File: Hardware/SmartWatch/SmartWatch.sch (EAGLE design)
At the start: 1 part

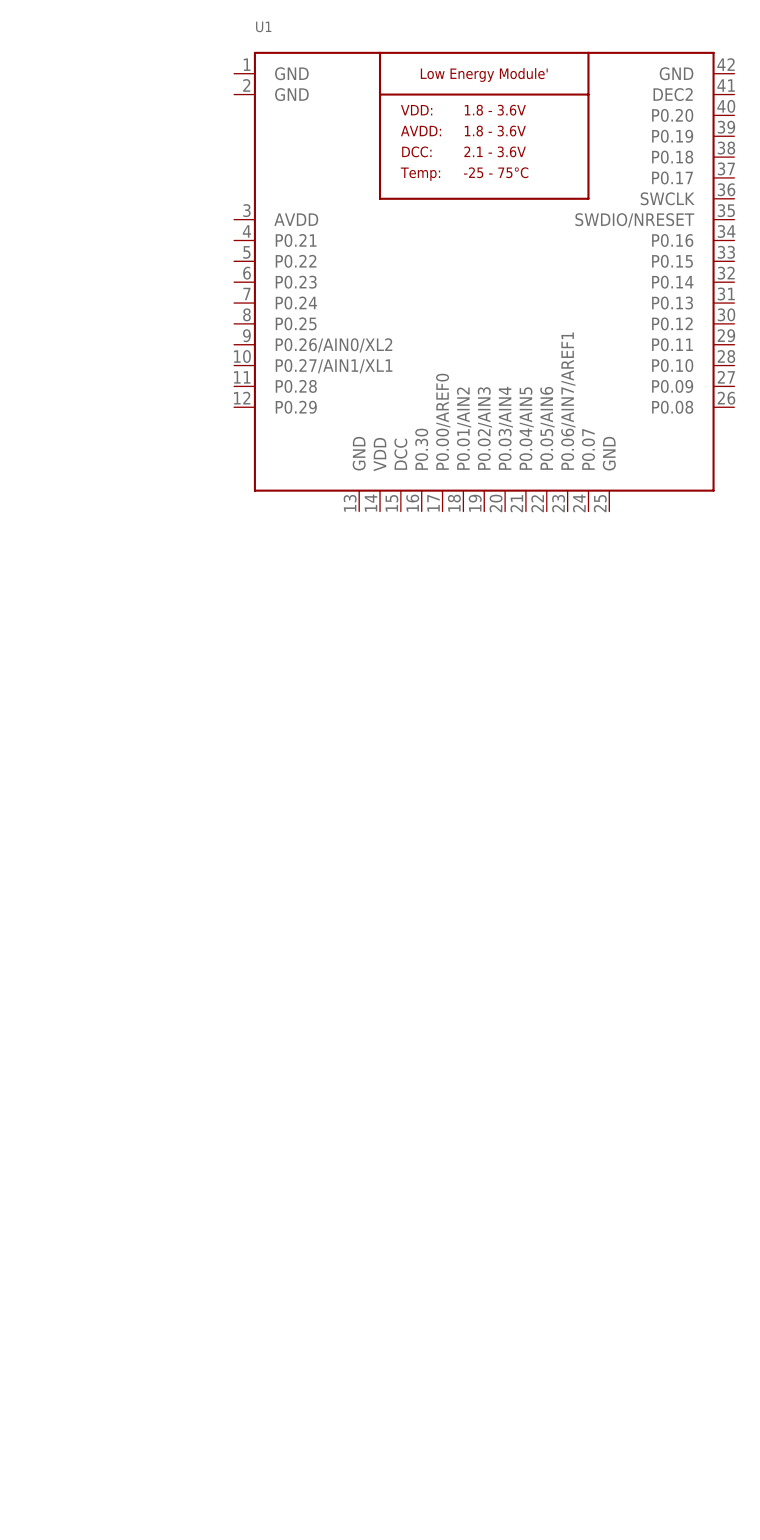
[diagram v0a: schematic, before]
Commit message: adding things to library
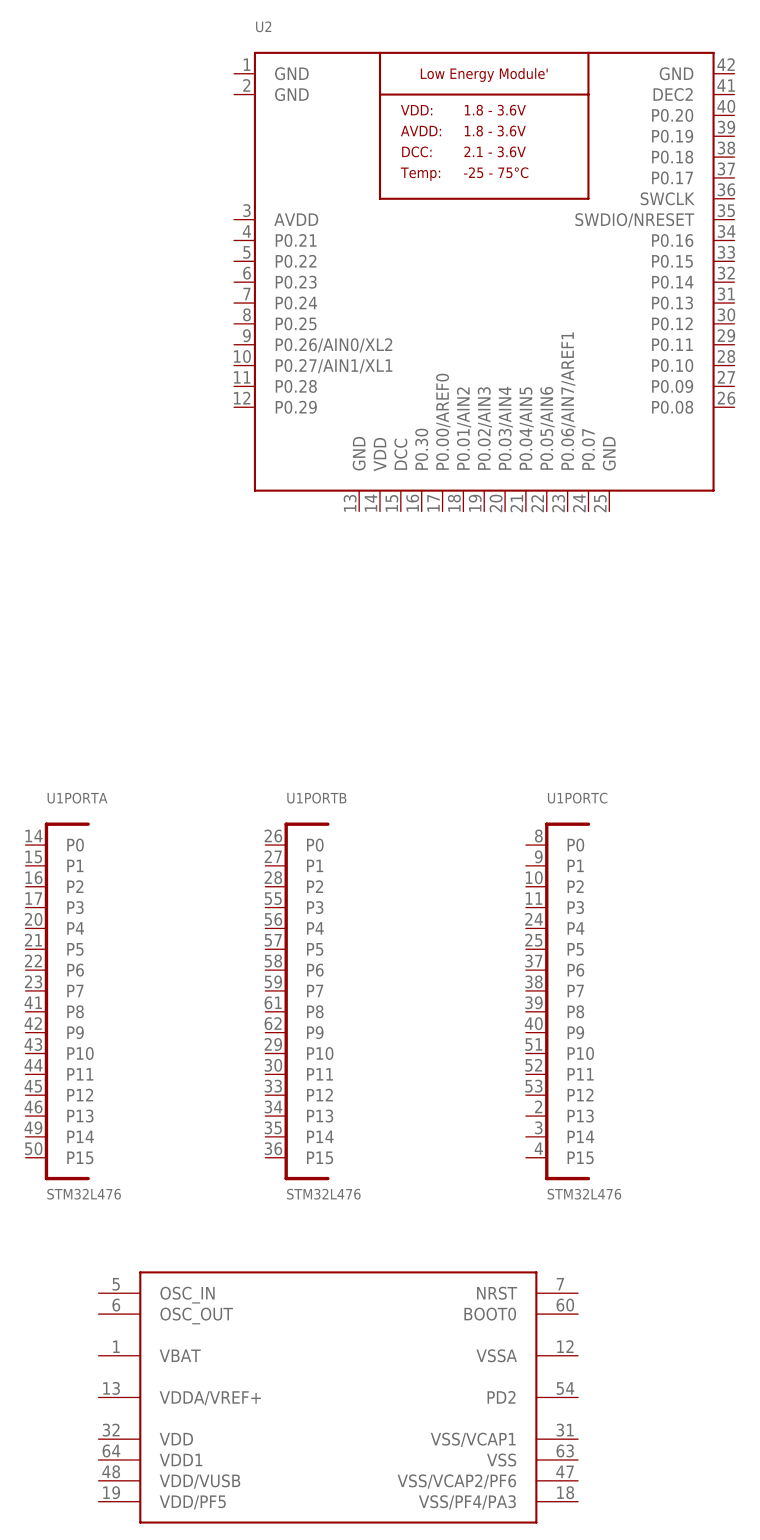
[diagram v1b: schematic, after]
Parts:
- added U2: (no value), SmartWatch:NRF51822_MODULE_MDBT40
- U1: value (none) -> STM32L476; device SmartWatch:NRF51822_MODULE_MDBT40 -> SmartWatch:STM32L476
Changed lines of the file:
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@@
 <setting verticaltext="up"/>
 </settings>
-<grid distance="0.1" unitdist="inch" unit="inch" style="lines" multiple="1" display="no" altdistance="0.01" altunitdist="inch" altunit="inch"/>
+<grid distance="0.05" unitdist="inch" unit="inch" style="lines" multiple="1" display="yes" altdistance="0.005" altunitdist="inch" altunit="inch"/>
 <layers>
 <layer number="1" name="Top" color="4" fill="1" visible="no" active="no"/>
@@
 </classes>
 <parts>
-<part name="U1" library="SmartWatch" deviceset="NRF51822_MODULE_MDBT40" device=""/>
+<part name="U2" library="SmartWatch" deviceset="NRF51822_MODULE_MDBT40" device=""/>
+<part name="U1" library="SmartWatch" deviceset="STM32L476" device=""/>
 </parts>
 <sheets>
@@
 </plain>
 <instances>
-<instance part="U1" gate="G$1" x="78.74" y="68.58"/>
+<instance part="U2" gate="G$1" x="78.74" y="68.58"/>
+<instance part="U1" gate="PORTA" x="27.94" y="-20.32"/>
+<instance part="U1" gate="PORTB" x="57.15" y="-20.32"/>
+<instance part="U1" gate="PORTC" x="88.9" y="-20.32"/>
+<instance part="U1" gate="G$4" x="57.15" y="-67.31"/>
 </instances>
 <busses>
